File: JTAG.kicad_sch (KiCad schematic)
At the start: 21 parts, among them U1 XC7Z020-1CLG400I__, U4 ATSHA204A-SSHCZ-T, U7 S25FL128SAGMFI000

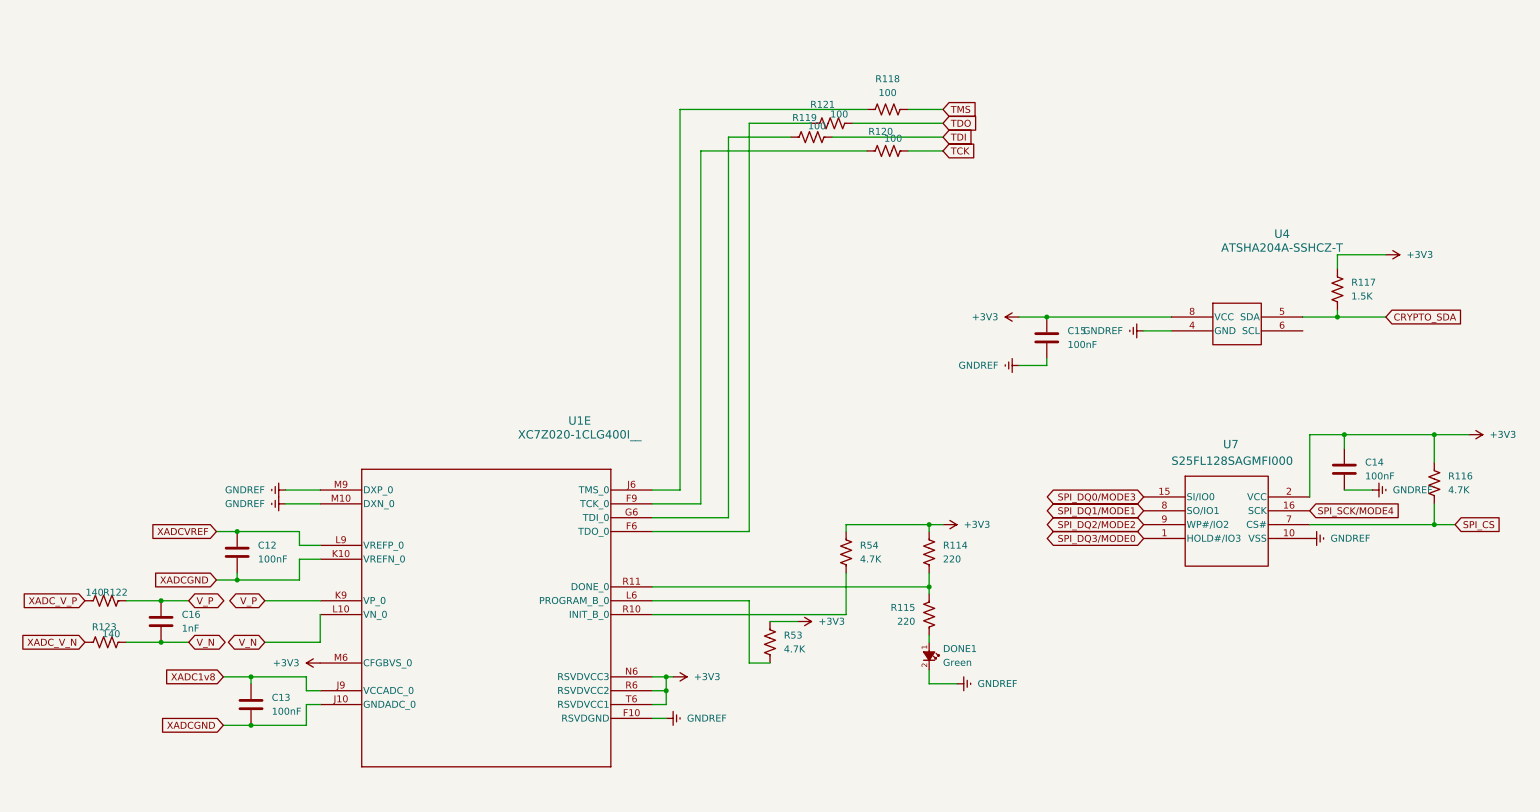
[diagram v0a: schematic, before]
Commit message: Layout update
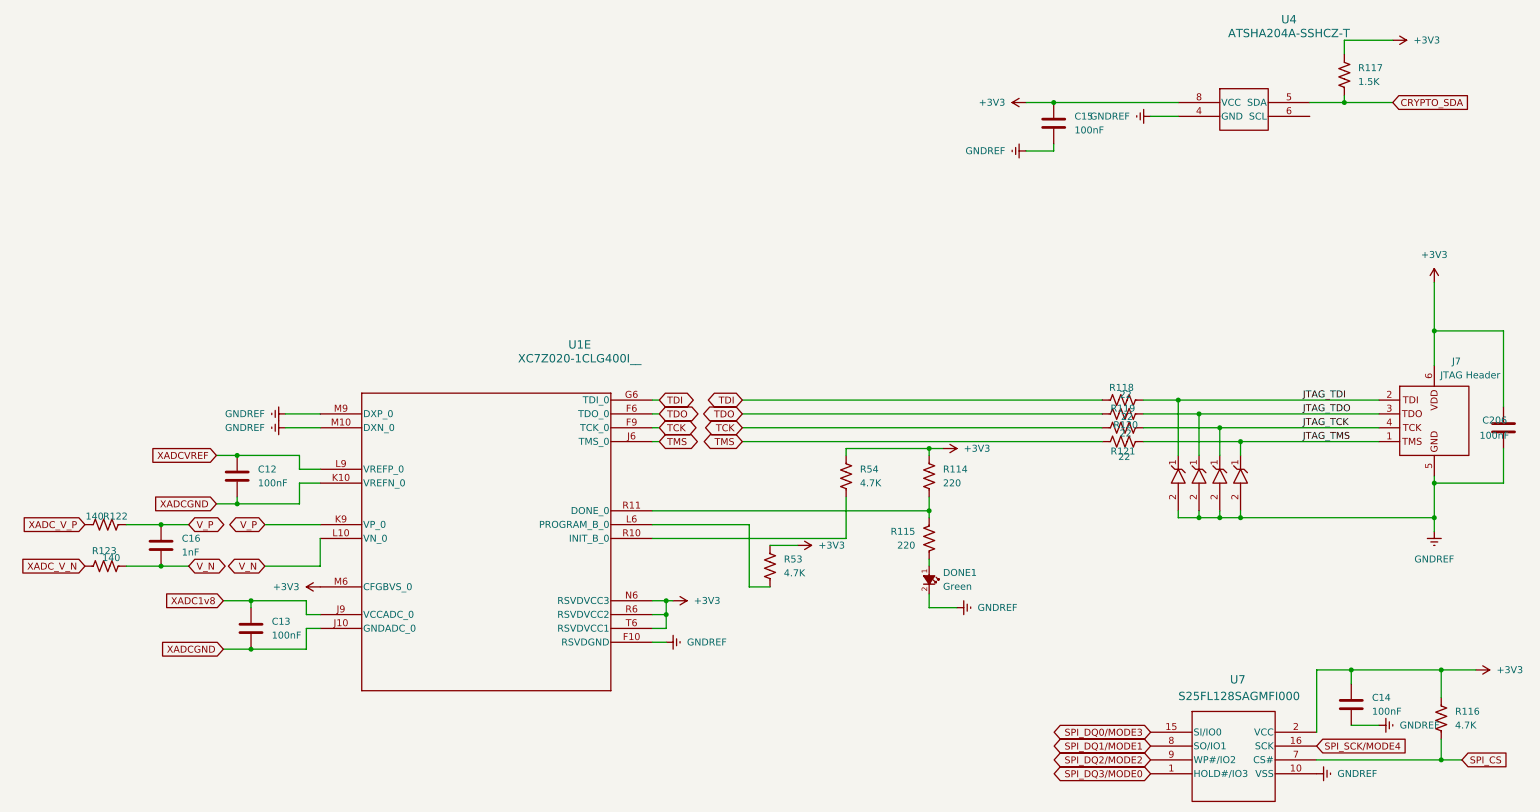
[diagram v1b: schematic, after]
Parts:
- added C206: 100nF, footprints:C_0201_0603Metric, symbol Device:C
- added J7: JTAG Header, footprints:PinHeader_1x06_P2.54mm_Vertical, symbol Connector:Conn_01x06_Pin
- added RV3, RV4, RV5, RV6: CG0402MLU-3.3G, footprints:VARC1005X41N, symbol CG0402MLU-3_3G:CG0402MLU-3.3G
- R118, R119, R120, R121: value 100 -> 22; footprint footprints:R_0402 -> footprints:R_0201_0603Metric; LCSC PN C106232 -> (none)
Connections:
- net +3V3: now also C206.1, J7.6 (VDD)
- net GNDREF: now also U7.3 (RESET#/RFU), C206.2, J7.5 (GND), RV3.2, RV4.2, RV5.2, RV6.2
- net TCK: now also R120.1, U1.F9 (TCK_0); no longer R120.2
- net TDI: now also R118.1, U1.G6 (TDI_0); no longer R119.2
- net TDO: now also R119.1, U1.F6 (TDO_0); no longer R121.2
- net TMS: now also R121.1, U1.J6 (TMS_0); no longer R118.2
- new net JTAG_TCK: J7.4 (TCK), R120.2, RV5.1
- new net JTAG_TDI: J7.2 (TDI), R118.2, RV3.1
- new net JTAG_TDO: J7.3 (TDO), R119.2, RV4.1
- new net JTAG_TMS: J7.1 (TMS), R121.2, RV6.1
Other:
- moved on the sheet: C12, C13, C14, C15, C16, DONE1, R114, R115, R116, R117, R122, R123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
